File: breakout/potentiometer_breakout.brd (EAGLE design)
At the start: 13 x 14.1 mm, 5 parts

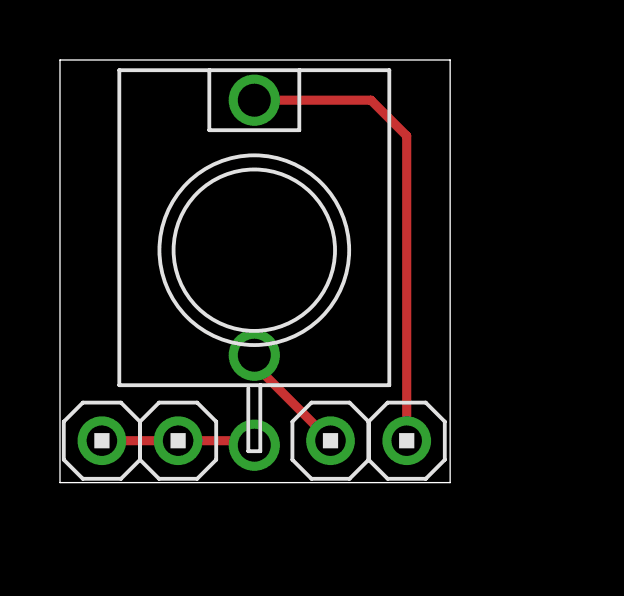
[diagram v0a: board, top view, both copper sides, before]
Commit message: Changes
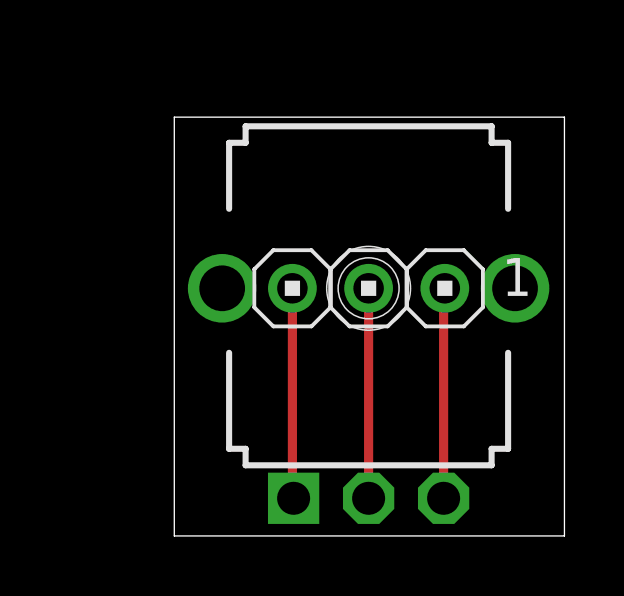
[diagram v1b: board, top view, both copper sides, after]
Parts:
- removed GND, GND1, NORM, SIG: HEADER/MALE/01, connectors:HEADER/MALE/01
- removed U$1: WQP-PJ301M-12_JACK, controls:WQP-PJ301M-12_JACK
- added 1, 2, 3: HEADER/MALE/01, connectors:HEADER/MALE/01
- added VR1: (no value), controls:9MM_SNAP-IN_POT
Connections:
- removed net N$6: GND.1, GND1.1, U$1.P$3
- new net N$3: 3.1, VR1.1
- net N$1: now also 1.1, VR1.3; no longer SIG.1, U$1.P$1
- net N$2: now also 2.1, VR1.2; no longer NORM.1, U$1.P$2
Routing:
- net N$1: track 15.7 -> 7.02 mm
- net N$3: track 0.00 -> 7.02 mm
- net N$6: track 5.14 -> 0.00 mm
- net N$2: track 3.90 -> 7.00 mm
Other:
- board size 13 x 14.1 mm -> 13 x 14 mm
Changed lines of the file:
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@@
 <setting verticaltext="up"/>
 </settings>
-<grid distance="50" unitdist="mil" unit="mil" style="lines" multiple="1" display="no" altdistance="10" altunitdist="mil" altunit="mil"/>
+<grid distance="50" unitdist="mil" unit="mil" style="lines" multiple="1" display="no" altdistance="5" altunitdist="mil" altunit="mil"/>
 <layers>
 <layer number="1" name="Top" color="4" fill="1" visible="yes" active="yes"/>
@@
 <board>
 <plain>
-<wire x1="2.413" y1="6.223" x2="15.418" y2="6.223" width="0" layer="20"/>
-<wire x1="15.418" y1="6.223" x2="15.418" y2="20.31" width="0" layer="20"/>
-<wire x1="15.418" y1="20.31" x2="2.413" y2="20.31" width="0" layer="20"/>
-<wire x1="2.413" y1="20.31" x2="2.413" y2="6.223" width="0" layer="20"/>
+<wire x1="6.223" y1="4.445" x2="19.228" y2="4.445" width="0" layer="20"/>
+<wire x1="19.228" y1="4.445" x2="19.228" y2="18.405" width="0" layer="20"/>
+<wire x1="19.228" y1="18.405" x2="6.223" y2="18.405" width="0" layer="20"/>
+<wire x1="6.223" y1="18.405" x2="6.223" y2="4.445" width="0" layer="20"/>
 </plain>
 <attributes>
@@
 </autorouter>
 <elements>
-<element name="GND" library="connectors" package="HEADER/MALE/01" value="HEADER/MALE/01" x="3.81" y="7.62" smashed="yes" rot="R90">
-<attribute name="NAME" x="4.572" y="9.525" size="1.016" layer="26" ratio="10" rot="MR90"/>
+<element name="2" library="connectors" package="HEADER/MALE/01" value="HEADER/MALE/01" x="12.7" y="12.7" smashed="yes"/>
+<element name="VR1" library="controls" package="9MM_SNAP-IN_POT" value="" x="12.7" y="12.7" smashed="yes">
+<attribute name="VALUE" x="8.89" y="8.89" size="1.27" layer="27"/>
 </element>
-<element name="NORM" library="connectors" package="HEADER/MALE/01" value="HEADER/MALE/01" x="11.43" y="7.62" smashed="yes" rot="R90">
-<attribute name="NAME" x="10.922" y="9.525" size="1.016" layer="26" ratio="10" rot="MR90"/>
+<element name="1" library="connectors" package="HEADER/MALE/01" value="HEADER/MALE/01" x="15.24" y="12.7" smashed="yes">
+<attribute name="NAME" x="17.145" y="12.446" size="1.27" layer="25" ratio="10"/>
 </element>
-<element name="SIG" library="connectors" package="HEADER/MALE/01" value="HEADER/MALE/01" x="13.97" y="7.62" smashed="yes" rot="R90">
-<attribute name="NAME" x="13.462" y="9.525" size="1.016" layer="26" ratio="10" rot="MR90"/>
-</element>
-<element name="U$1" library="controls" package="WQP-PJ301M-12_JACK" value="WQP-PJ301M-12_JACK" x="8.89" y="13.97" smashed="yes"/>
-<element name="GND1" library="connectors" package="HEADER/MALE/01" value="HEADER/MALE/01" x="6.35" y="7.62" smashed="yes"/>
+<element name="3" library="connectors" package="HEADER/MALE/01" value="HEADER/MALE/01" x="10.16" y="12.7" smashed="yes"/>
 </elements>
 <signals>
 <signal name="N$1">
-<contactref element="U$1" pad="P$1"/>
-<contactref element="SIG" pad="1"/>
-<wire x1="13.97" y1="7.62" x2="13.97" y2="17.78" width="0.3048" layer="1"/>
-<wire x1="13.97" y1="17.78" x2="12.78" y2="18.97" width="0.3048" layer="1"/>
-<wire x1="12.78" y1="18.97" x2="8.89" y2="18.97" width="0.3048" layer="1"/>
+<contactref element="VR1" pad="3"/>
+<contactref element="1" pad="1"/>
+<wire x1="15.2" y1="5.7" x2="15.2" y2="12.66" width="0.3048" layer="1"/>
+<wire x1="15.2" y1="12.66" x2="15.24" y2="12.7" width="0.3048" layer="1"/>
 </signal>
 <signal name="N$2">
-<contactref element="U$1" pad="P$2"/>
-<contactref element="NORM" pad="1"/>
-<wire x1="11.43" y1="7.62" x2="8.89" y2="10.16" width="0.3048" layer="1"/>
-<wire x1="8.89" y1="10.16" x2="8.89" y2="10.47" width="0.3048" layer="1"/>
+<contactref element="VR1" pad="2"/>
+<contactref element="2" pad="1"/>
+<wire x1="12.7" y1="12.7" x2="12.7" y2="5.7" width="0.3048" layer="1"/>
 </signal>
-<signal name="N$6">
-<contactref element="U$1" pad="P$3"/>
-<contactref element="GND" pad="1"/>
-<contactref element="GND1" pad="1"/>
-<wire x1="3.81" y1="7.62" x2="6.35" y2="7.62" width="0.3048" layer="1"/>
-<wire x1="6.35" y1="7.62" x2="8.74" y2="7.62" width="0.3048" layer="1"/>
-<wire x1="8.74" y1="7.62" x2="8.89" y2="7.47" width="0.3048" layer="1"/>
+<signal name="N$3">
+<contactref element="VR1" pad="1"/>
+<contactref element="3" pad="1"/>
+<wire x1="10.2" y1="5.7" x2="10.16" y2="5.74" width="0.3048" layer="1"/>
+<wire x1="10.16" y1="5.74" x2="10.16" y2="12.7" width="0.3048" layer="1"/>
 </signal>
 </signals>
